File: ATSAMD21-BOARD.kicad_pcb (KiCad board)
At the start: 4 copper layers, 45 x 70 mm, 82 parts, among them J1 J-LINK, J2 BATT, J3 CON_USB_GCT_USB4105_REVA, J5 ROW, J6 COL, J7 EXPOSED, M1 MNT, M2 MNT, M3 MNT, Q1 P-MOSFET-MIC94052, SW1 RST, SW2 RST, U1 ATSAMD21G17D-A, U10 DA14531MOD-00F01002, U12 IS31FL3737, U2 TLV70245_SOT23-5, U3 TLV70245_SOT23-5, U4 RF_LORA_RFM95W-915S2, U5 MCP73831-2-OT, U6 16MB-W25Q16JVSNIQ, U7 CH340C, U8 IC-SENSOR-TEMP-HUM-SHT4X, U9 TLV70245_SOT23-5, Y1 12MHz

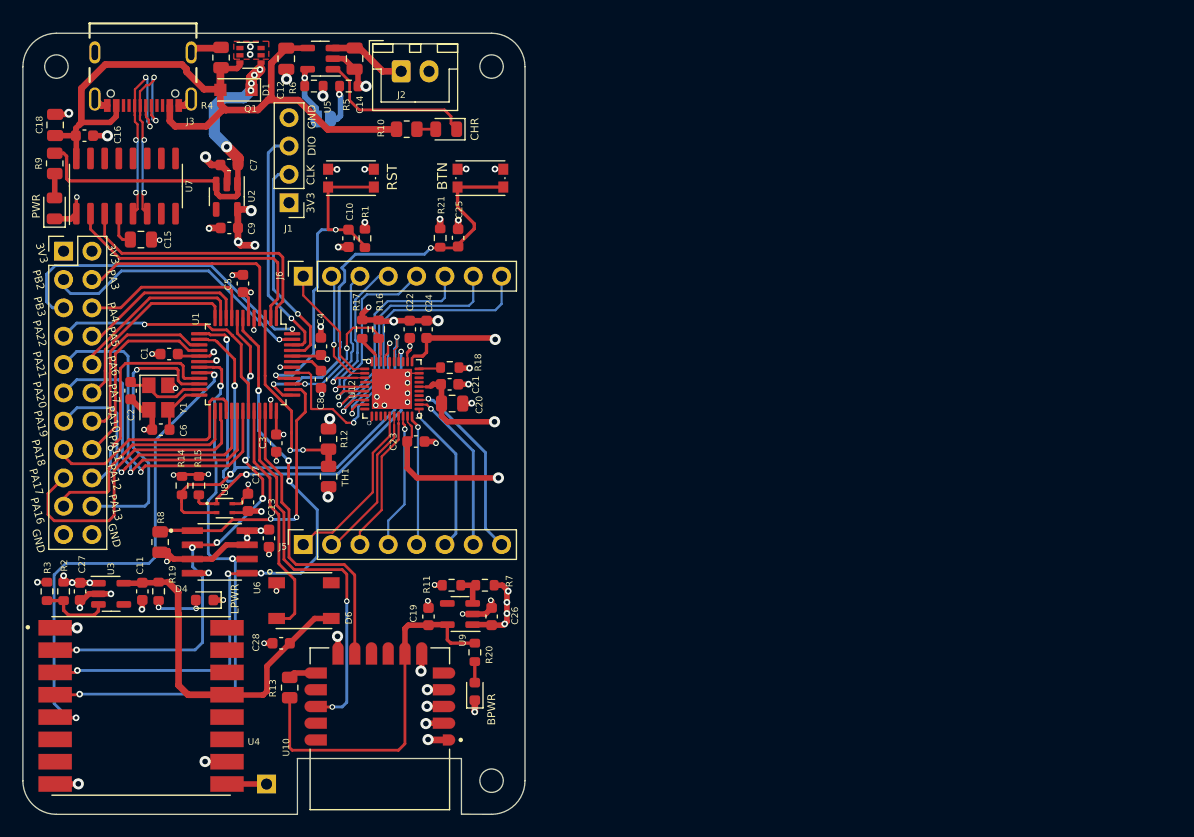
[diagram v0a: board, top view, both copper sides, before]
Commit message: Update the design
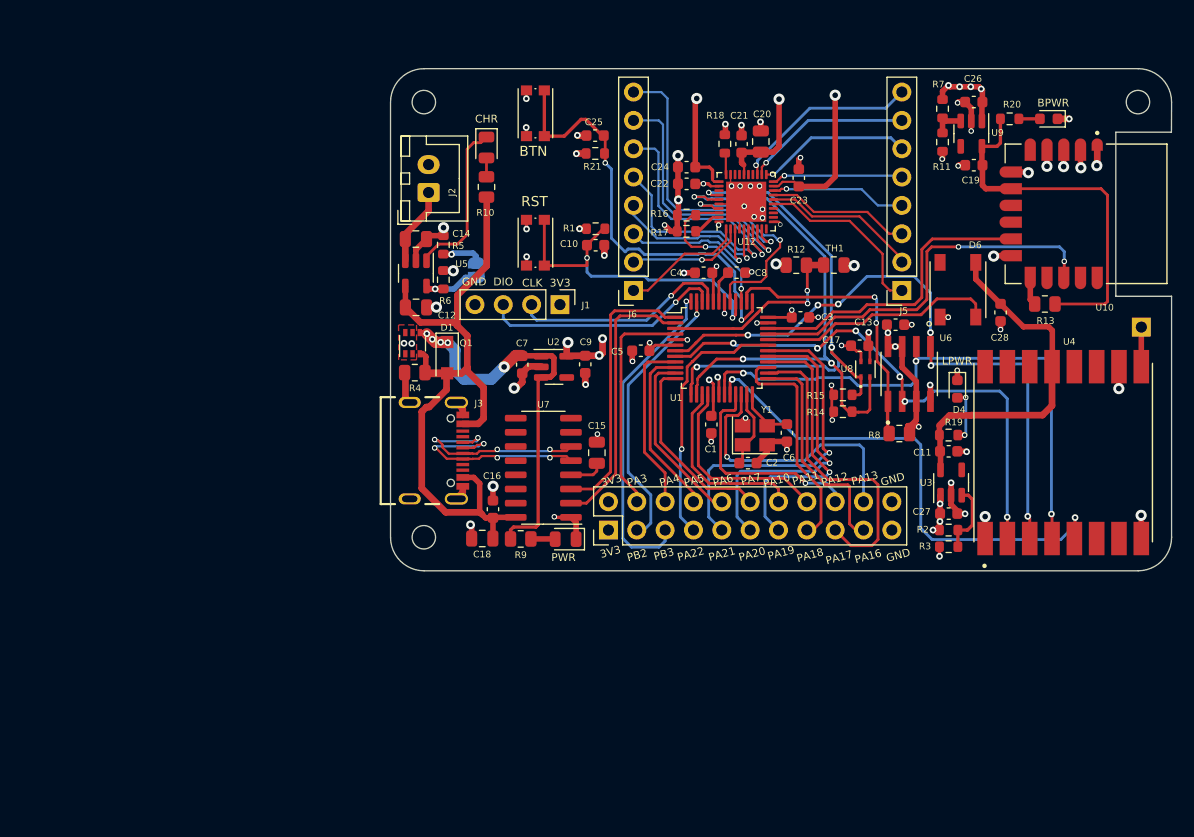
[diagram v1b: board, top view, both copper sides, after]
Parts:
- moved AE1 88.5 mm to (187.2, 89.3), turned to 180 degrees
- moved U4 85.7 mm to (180.2, 100.6), turned to 90 degrees
- moved M3 84.0 mm to (186.9, 69.2), turned to 90 degrees
- moved R3 80.9 mm to (170.0, 109.0), turned to 180 degrees
- moved R2 79.5 mm to (170.0, 107.5), turned to 0 degrees
- moved U10 78.3 mm to (182.3, 79.2), turned to -90 degrees
- moved C27 78.2 mm to (170.0, 106.0), turned to 0 degrees
- moved U3 75.9 mm to (170.2, 103.3), turned to 90 degrees
- moved R13 75.9 mm to (178.6, 87.3), turned to 180 degrees
- moved C11 73.3 mm to (170.0, 100.5), turned to 0 degrees
- moved D5 72.7 mm to (178.9, 70.7), turned to 180 degrees
- moved R19 72.2 mm to (170.0, 99.0), turned to 0 degrees
- moved C28 71.0 mm to (174.6, 88.0), turned to -90 degrees
- moved D4 70.1 mm to (170.8, 94.9), turned to -90 degrees
- moved R20 67.7 mm to (175.4, 70.7), turned to 0 degrees
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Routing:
- net Net-(J5-Pad5): track 13.9 -> 12.4 mm
- net Net-(J5-Pad1): track 15.6 -> 16.3 mm
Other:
- board size 45 x 70 mm -> 70 x 45 mm
